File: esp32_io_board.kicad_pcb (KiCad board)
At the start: 2 copper layers, 58 x 49 mm, 55 parts, among them J1 USB_B_Micro, J11 Conn_01x02, J12 Conn_01x02, J14 Conn_01x02, J18 Conn_01x02, J2 Conn_02x04_Counter_Clockwise, J3 Conn_01x02, J5 RASPBERRYPI-40-PIN-GPIO, J7 Conn_01x02, SW1 Reset, SW2 Bootloader, U1 CP2102N-A01-GQFN24, U2 TXB0104PW, U3 TXB0104PW, U4 ESP32-WROOM, U5 LM1117-3.3, U6 TCA9548APWR

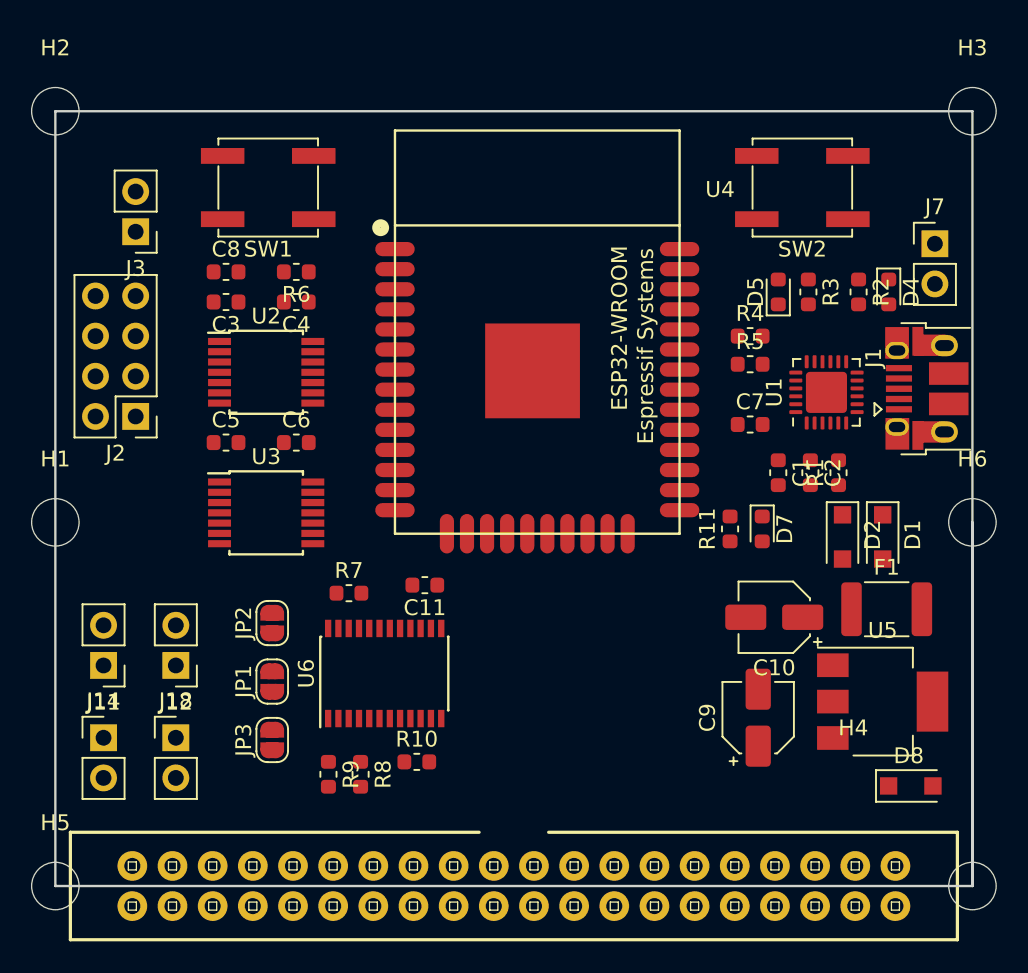
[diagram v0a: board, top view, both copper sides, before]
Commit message: layout
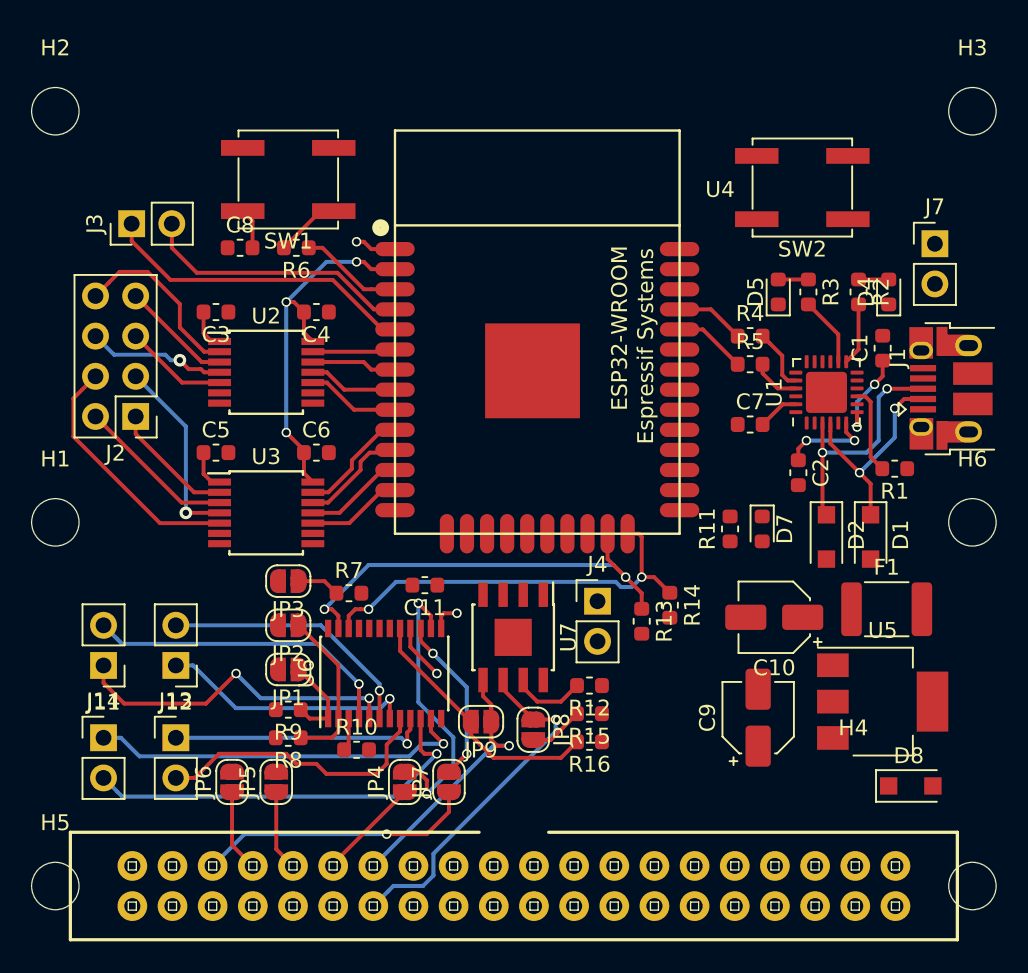
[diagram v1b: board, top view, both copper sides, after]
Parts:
- removed J18: Conn_01x02, Connector_PinHeader_2.54mm:PinHeader_1x02_P2.54mm_Vertical
- added J13: Conn_01x02, Connector_PinHeader_2.54mm:PinHeader_1x02_P2.54mm_Vertical, F.Cu at (167.6, 120.9)
- added J4: Conn_01x02, Connector_PinHeader_2.54mm:PinHeader_1x02_P2.54mm_Vertical, F.Cu at (194.3, 112.3)
- added JP4: SolderJumper_2_Open, Jumper:SolderJumper-2_P1.3mm_Open_RoundedPad1.0x1.5mm, F.Cu at (182.1, 123.7)
- added JP5: SolderJumper_2_Open, Jumper:SolderJumper-2_P1.3mm_Open_RoundedPad1.0x1.5mm, F.Cu at (174.0, 123.7)
- added JP6: SolderJumper_2_Open, Jumper:SolderJumper-2_P1.3mm_Open_RoundedPad1.0x1.5mm, F.Cu at (171.2, 123.7)
- added JP7: SolderJumper_2_Open, Jumper:SolderJumper-2_P1.3mm_Open_RoundedPad1.0x1.5mm, F.Cu at (184.9, 123.7)
- added JP8: SolderJumper_2_Open, Jumper:SolderJumper-2_P1.3mm_Open_RoundedPad1.0x1.5mm, F.Cu at (190.2, 120.4)
- added JP9: SolderJumper_2_Open, Jumper:SolderJumper-2_P1.3mm_Open_RoundedPad1.0x1.5mm, F.Cu at (186.9, 119.9)
- added R12: R_Small, Resistor_SMD:R_0603_1608Metric, F.Cu at (193.8, 117.6)
- added R13: R_Small, Resistor_SMD:R_0603_1608Metric, F.Cu at (197.1, 113.5)
- added R14: R_Small, Resistor_SMD:R_0603_1608Metric, F.Cu at (198.9, 112.5)
- added R15: R_Small, Resistor_SMD:R_0603_1608Metric, F.Cu at (193.8, 119.4)
- added R16: R_Small, Resistor_SMD:R_0603_1608Metric, F.Cu at (193.8, 121.2)
- added U7: CAT24C256, Package_SO:SOIC-8-1EP_3.9x4.9mm_P1.27mm_EP2.35x2.35mm, F.Cu at (189.0, 114.6)
- moved C1 10.3 mm to (212.3, 96.3), turned to 90 degrees
- moved JP3 10.1 mm to (174.8, 111.0), turned to 180 degrees
- moved R8 5.12 mm to (174.8, 120.9), turned to 180 degrees
- moved R9 4.81 mm to (174.8, 119.1), turned to 180 degrees
- moved R10 3.89 mm to (179.1, 121.7)
- moved R1 3.57 mm to (213.1, 103.9), turned to 180 degrees
- moved C8 1.76 mm to (171.7, 89.9)
- moved J1 1.52 mm to (216.7, 98.8)
- moved R6 1.52 mm to (175.3, 89.9)
- moved C4 1.42 mm to (176.5, 94.0)
- moved C6 1.42 mm to (176.5, 102.9)
- moved SW1 1.37 mm to (174.8, 85.6)
- moved JP1 1.27 mm to (174.8, 116.6), turned to 180 degrees
- moved JP2 1.03 mm to (174.8, 113.8), turned to 180 degrees
- moved D2 1.02 mm to (208.8, 108.2)
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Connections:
- C6 pad 1: 3.3V -> +3V3
- J5 pad 27: Net-(J5-Pad27) -> /id_sda
- J5 pad 28: Net-(J5-Pad28) -> /id_clk
- U4 pad 14: /di -> Net-(J4-Pad2)
- U4 pad 16: /ci -> Net-(J4-Pad1)
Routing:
- net +3V3: track 0.00 -> 35.3 mm, vias 0 -> 7
- net Net-(R13-Pad1): track 0.00 -> 28.5 mm, vias 0 -> 2
- net Net-(R14-Pad1): track 0.00 -> 26.3 mm, vias 0 -> 2
- net Net-(J14-Pad2): track 0.00 -> 25.8 mm, vias 0 -> 1
- net Net-(J14-Pad1): track 0.00 -> 24.2 mm, vias 0 -> 1
- net /id_clk: track 0.00 -> 22.4 mm, vias 0 -> 1
- net Net-(J11-Pad1): track 0.00 -> 21.2 mm, vias 0 -> 2
- net Net-(J11-Pad2): track 0.00 -> 20.3 mm, vias 0 -> 1
- net Net-(J3-Pad1): track 0.00 -> 20.1 mm
- net Net-(JP4-Pad2): track 0.00 -> 18.1 mm, vias 0 -> 2
- net Net-(J13-Pad2): track 0.00 -> 18.0 mm
- net Net-(J5-Pad35): track 0.00 -> 17.6 mm, vias 0 -> 1
- net Net-(J3-Pad2): track 0.00 -> 17.3 mm
- net /id_sda: track 0.00 -> 17.0 mm, vias 0 -> 1
- net Net-(J12-Pad2): track 0.00 -> 16.6 mm, vias 0 -> 1
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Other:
- board outline removed
- net class Default: via_dia 0.8 -> 0.6
